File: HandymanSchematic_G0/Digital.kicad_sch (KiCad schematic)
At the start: 31 parts, among them J1 SWD Header, J2 PWR, J3 JACKS, J4 FOOTSWITCH, J5 ScopeGroundLoop, Q2 2N7002, Q3 2N7002, SW1 RST, SW2 BYP, U3 STM32G030F6P6, U4 AMS1117, U5 SSD1306

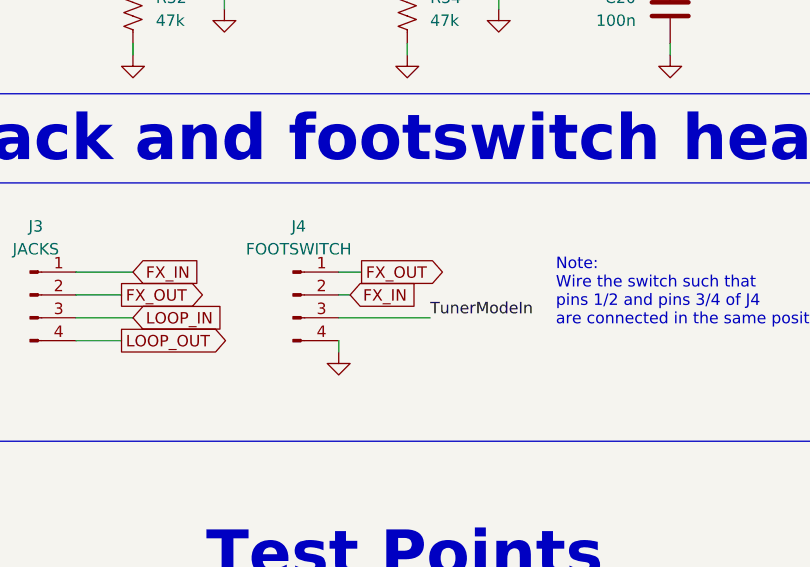
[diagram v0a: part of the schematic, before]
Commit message: routed, DRC passing
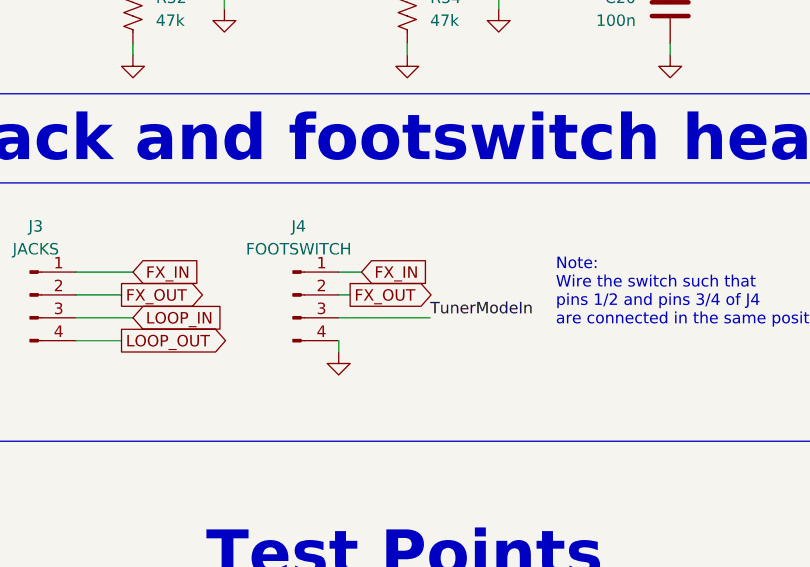
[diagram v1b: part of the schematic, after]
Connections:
- net FX_IN: now also J4.1 (Pin_1); no longer J4.2 (Pin_2)
- net FX_OUT: now also J4.2 (Pin_2); no longer J4.1 (Pin_1)
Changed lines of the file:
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@@
 	(global_label "FX_IN"
 		(shape input)
-		(at 191.77 99.06 0)
+		(at 193.04 96.52 0)
 		(fields_autoplaced yes)
 		(effects
@@
 		)
 		(property "Intersheetrefs" "${INTERSHEET_REFS}"
-			(at 199.9562 99.06 0)
+			(at 201.2262 96.52 0)
 			(effects
 				(font
@@
 	(global_label "FX_OUT"
 		(shape output)
-		(at 193.04 96.52 0)
+		(at 191.77 99.06 0)
 		(fields_autoplaced yes)
 		(effects
@@
 		)
 		(property "Intersheetrefs" "${INTERSHEET_REFS}"
-			(at 202.9195 96.52 0)
+			(at 201.6495 99.06 0)
 			(effects
 				(font
